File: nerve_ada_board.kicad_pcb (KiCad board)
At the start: 4 copper layers, 120 x 120 mm, 64 parts, among them J10 PC1-3, J11 PB4-5, J2 TC2050-IDC, J3 2171750001, J5 WS2812B, J6 Camera, J7 CAN1, J8 CAN2, J9 PA4-7, SW1 SPST, SW2 SPST, SW3 SPST, U1 LD1117S33TR_SOT223, U2 STM32F446RET, U3 SAM-M10Q, U4 XBP9B-DMWT-002, U8 TXB0104QPWRQ1, U9 TXB0104QPWRQ1, Y1 8M, Y2 32k768

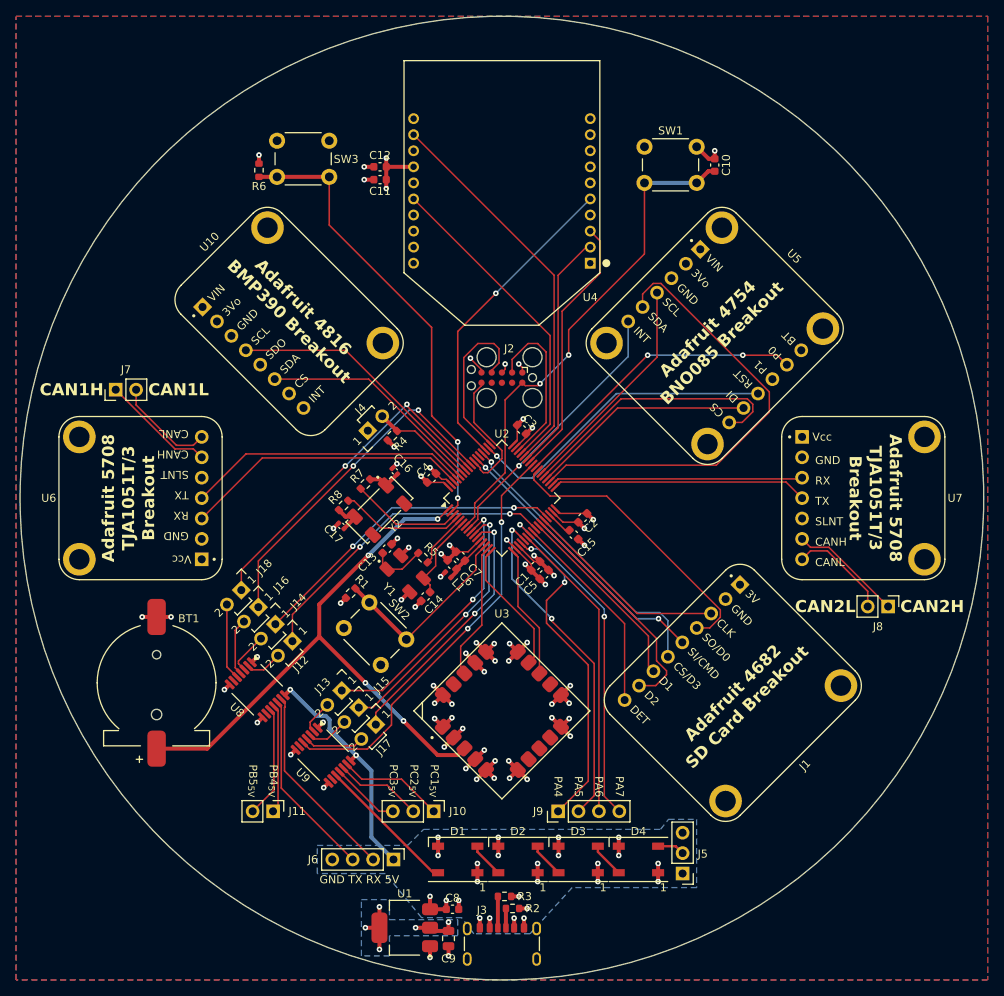
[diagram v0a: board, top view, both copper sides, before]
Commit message: Flight ready alpha and update components
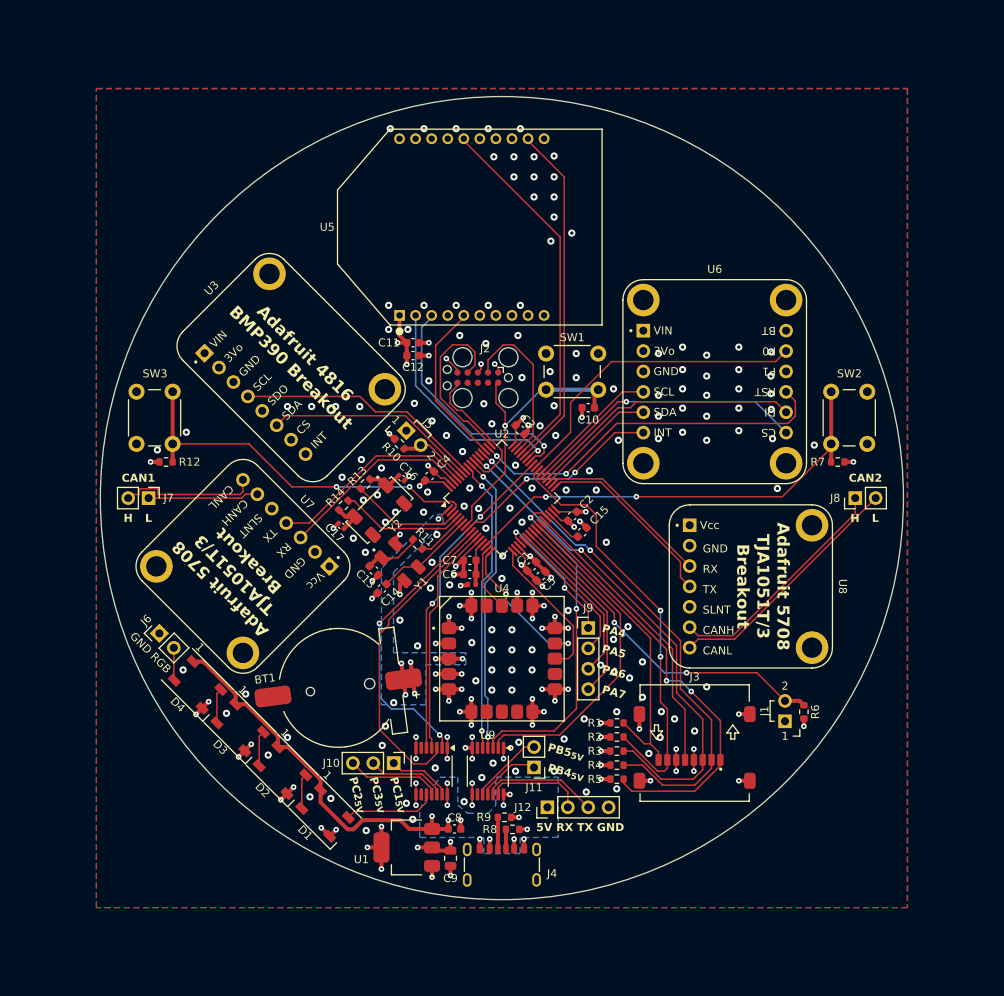
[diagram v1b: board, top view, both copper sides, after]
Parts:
- removed the J12 at (121.5, 123.7)
- removed J13, J14, J15, J16, J17, J18: ~, common:harwin_2p_2-54_jumper_closed
- removed the J5 at (171.0, 151.8)
- added J3: 472192001, common:molex_472192001_microsd_hinge, F.Cu at (172.5, 135.5)
- added J6: WS2812B, Connector_PinHeader_2.54mm:PinHeader_1x02_P2.54mm_Vertical, F.Cu at (105.8, 121.8)
- added R1: 47k, Resistor_SMD:R_0603_1608Metric, F.Cu at (162.8, 133.0)
- added R2: 47k, Resistor_SMD:R_0603_1608Metric, F.Cu at (162.8, 134.8)
- added R3: 47k, Resistor_SMD:R_0603_1608Metric, F.Cu at (162.8, 136.5)
- added R4: 47k, Resistor_SMD:R_0603_1608Metric, F.Cu at (162.8, 138.2)
- added R5: 47k, Resistor_SMD:R_0603_1608Metric, F.Cu at (162.8, 140.0)
- added R6: 10k, Resistor_SMD:R_0603_1608Metric, F.Cu at (186.1, 131.6)
- J1: footprint adafruit:adafruit_4682_sdio_card -> common:harwin_2p_2-54_jumper_open
- moved R7 62.8 mm to (190.3, 100.5), turned to 180 degrees
- moved SW2 60.8 mm to (189.5, 98.2), turned to 90 degrees
- moved D4 59.0 mm to (110.6, 128.3), turned to -45 degrees
- moved D3 45.2 mm to (115.9, 133.6), turned to -45 degrees
- moved SW3 41.6 mm to (103.0, 98.2), turned to 90 degrees
- moved R12 38.1 mm to (106.7, 100.5), turned to 0 degrees
- moved C10 34.1 mm to (159.2, 93.8), turned to 0 degrees
- moved J11 33.0 mm to (152.5, 138.5), turned to 180 degrees
- moved D2 31.4 mm to (121.2, 138.9), turned to -45 degrees
- moved U9 30.5 mm to (146.8, 139.0), turned to -90 degrees
- moved SW1 28.5 mm to (154.0, 87.0)
- moved C12 23.9 mm to (137.4, 87.3), turned to 0 degrees
- moved J9 23.1 mm to (159.2, 121.2), turned to 0 degrees
- moved BT1 22.6 mm to (128.1, 128.6), turned to 97.5 degrees
- moved C11 20.7 mm to (137.4, 85.7), turned to 0 degrees
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- renumbered J6 to J12, J3 to J4, J4 to J5, R4 to R10, R5 to R11, R6 to R12, R7 to R13, R8 to R14, R1 to R7, R2 to R8, R3 to R9, U9 to U10, U10 to U3, U3 to U4, U4 to U5, U5 to U6, U6 to U7, U7 to U8, U8 to U9
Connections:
- J1 pad 2: GND -> /SDIO_DET
- U10 pad 2: Net-(U9-A1) -> /PC1
- U10 pad 3: Net-(U9-A2) -> /PC2
- U10 pad 4: Net-(U9-A3) -> /PC3
- U9 pad 2: Net-(U8-A1) -> /USART3_RX
- U9 pad 3: Net-(U8-A2) -> /USART3_TX
- U9 pad 4: Net-(U8-A3) -> /PB4
- U9 pad 5: Net-(U8-A4) -> /PB5
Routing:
- net +3.3VBATT: track 75.6 -> 14.0 mm, vias 4 -> 7
- net /SPI2_MISO: track 57.0 -> 15.2 mm
- net Net-(U2-PA0): track 24.7 -> 57.4 mm, vias 0 -> 2
- net /SDIO_CMD: track 35.1 -> 63.1 mm
- net /SDIO_D3: track 36.9 -> 64.7 mm, vias 1 -> 2
- net /NRST: track 63.0 -> 36.4 mm, vias 2 -> 1
- net /SDIO_D2: track 29.3 -> 54.7 mm, vias 0 -> 2
- net /PA5: track 42.1 -> 18.0 mm, vias 2 -> 0
- net /PA4: track 41.1 -> 17.4 mm
- net /GPIO_RADIO_RST: track 39.6 -> 20.6 mm, vias 1 -> 0
- net /PA7: track 42.6 -> 24.2 mm, vias 2 -> 0
- net /CAN2-: track 12.6 -> 30.9 mm
- net /SDIO_DET: track 25.7 -> 43.4 mm, vias 0 -> 2
- net /SDIO_D0: track 35.8 -> 53.5 mm, vias 0 -> 2
- net /PA6: track 37.8 -> 21.1 mm
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- added copper zone on B.Cu, net +3.3VBATT
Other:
- board size 120 x 120 mm -> 100 x 100 mm
- board text added: "5V RX TX GND"
- board text added: "CAN1"
- board text added: "CAN2"
- board text added: "GND RGB"
- board text added: "H"
- board text added: "L"
- board text removed: "CAN1H"
- board text removed: "CAN1L"
- board text removed: "CAN2H"
- board text removed: "CAN2L"
- board text removed: "GND TX RX 5V"
